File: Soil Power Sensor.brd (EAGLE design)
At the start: 100 x 90 mm, 97 parts, among them IC1 TPD2E2U06DCK, J1 12401832E402A, U1 WIO E5, U10 FSA2466, U12 REF2033, U13 TLV1117LV33, U2 FT234XD, U3 MAX9943ATT+, U4 ESP32-C3-MINI-1-N4, U5 THS4532, U6 LM27761DSG, U7 INA296A5, U8 MAX11201A, X1 SMA-142-0701-801/806

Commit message: Reset board layout
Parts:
- moved C12 216.9 mm to (-105.4, 104.1), turned to 0 degrees
- moved C11 215.2 mm to (-102.9, 116.8), turned to 0 degrees
- moved R27 204.2 mm to (-97.8, 116.8), turned to 0 degrees
- moved R25 203.9 mm to (-87.6, 116.8), turned to 0 degrees
- moved J1 201.6 mm to (-91.4, 7.62), turned to 0 degrees
- moved R15 200.2 mm to (-106.7, 111.8), turned to 0 degrees
- moved R4 199.0 mm to (-101.6, 111.8), turned to 0 degrees
- moved R26 196.2 mm to (-92.7, 116.8), turned to 0 degrees
- moved R24 195.1 mm to (-82.5, 116.8), turned to 0 degrees
- moved TP5 191.9 mm to (-90.2, 120.7)
- moved R23 190.5 mm to (-77.5, 116.8), turned to 0 degrees
- moved C4 186.7 mm to (-91.4, 111.8), turned to 0 degrees
- moved R22 184.0 mm to (-72.4, 116.8), turned to 0 degrees
- moved C7 176.3 mm to (-96.5, 111.8), turned to 0 degrees
- moved JP7 174.4 mm to (-71.1, 86.4), turned to 0 degrees
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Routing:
- net +3V3: track 282.9 -> 0.00 mm, vias 10 -> 0
- net VCC: track 165.2 -> 0.00 mm, vias 4 -> 0
- net N$22: track 95.2 -> 0.00 mm
- net PB3/RTS/JTDO: track 88.2 -> 0.00 mm, vias 2 -> 0
- net PC1: track 79.3 -> 0.00 mm, vias 3 -> 0
- net PC0: track 74.8 -> 0.00 mm, vias 3 -> 0
- net PB4/CTS/JNTRST: track 68.9 -> 0.00 mm, vias 2 -> 0
- net VUSB: track 68.9 -> 0.00 mm, vias 3 -> 0
- net -3V3: track 68.2 -> 0.00 mm, vias 2 -> 0
- net ESP32_TXD0: track 61.6 -> 0.00 mm, vias 2 -> 0
- net ESP32_RXD0: track 60.0 -> 0.00 mm, vias 2 -> 0
- net JTCK: track 47.9 -> 0.00 mm
- net ESP32_NRST: track 45.7 -> 0.00 mm
- net ESP32_EN: track 45.4 -> 0.00 mm, vias 2 -> 0
- net JTMS: track 45.0 -> 0.00 mm
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- removed copper zone on layer 1, net GND
- removed copper zone on layer 15, net GND
- removed copper zone on layer 16, net GND
- removed copper zone on layer 2, net GND
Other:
- board size 100 x 90 mm -> 160 x 100 mm

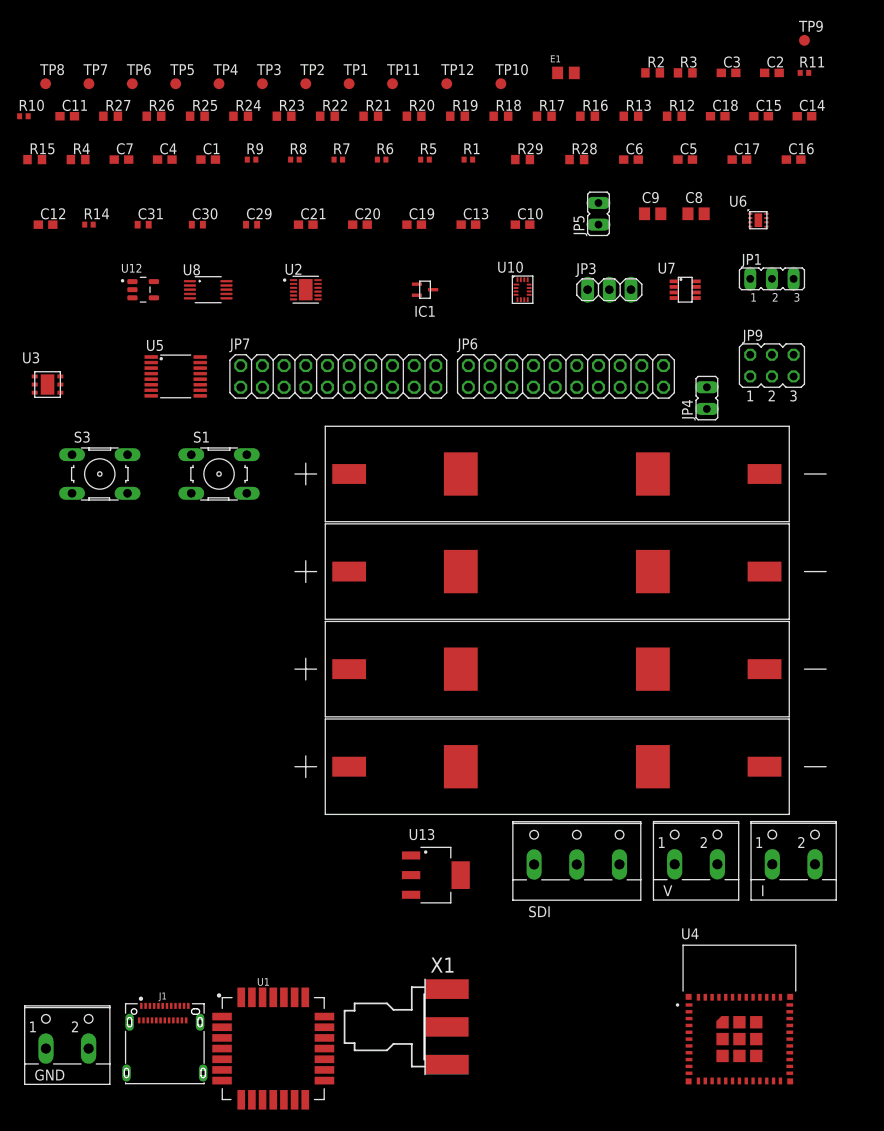
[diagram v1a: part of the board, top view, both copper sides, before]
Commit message: Renumbered all parts
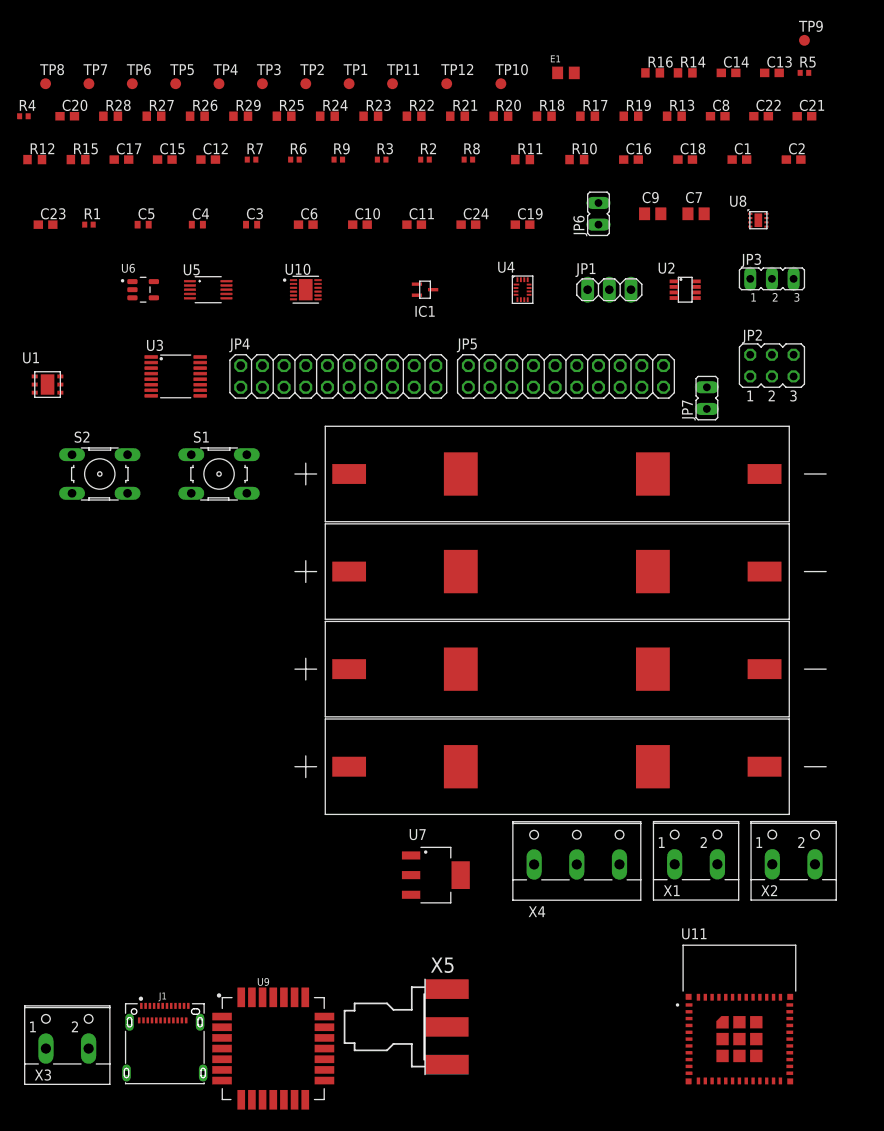
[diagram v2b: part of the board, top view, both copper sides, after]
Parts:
- removed C29, C30, C31: 0.1uF, rcl:C0402
- removed U12: REF2033, Soil Power Sensor:SOT95P280X110-5N
- removed U13: TLV1117LV33, Soil Power Sensor:SOT230P700X180-4N
- removed V: Voltage, con-wago-500:W237-102
- added C22: NC, rcl:C0603
- added C23: 10uF, rcl:C0603
- added C24: 0.1uF, rcl:C0603
- added U11: ESP32-C3-MINI-1-N4, Soil Power Sensor:XCVR_ESP32-C3-MINI-1-N4
- added U9: WIO E5, Soil Power Sensor:MODULE28P-1.25-12X12X2.5MM
- added X5: SMA-142-0701-801/806, con-coax:J502-ND-142-0701-801/806
- C1: value 4.7u -> 16uF
- C10: value 0.1uF -> 4.7uF
- C11: value 1uF -> 2.2uF
- C12: value 10uF -> 4.7u
- C13: value 0.1uF -> NC
- C15: value NC -> 0.1u
- C16: value 20uF -> 100n
- C17: value 16uF -> 4.7u
- C18: value 1uF -> 100n
- C19: value 2.2uF -> 0.1uF
- C2: value NC -> 20uF
- C20: value 4.7uF -> 1uF
- C21: value 4.7uF -> NC
- C3: value NC -> 0.1uF; device rcl:C0603 -> rcl:C0402
- C4: value 0.1u -> 0.1uF; device rcl:C0603 -> rcl:C0402
- C5: value 100n -> 0.1uF; device rcl:C0603 -> rcl:C0402
- C6: value 100n -> 4.7uF
- C7: value 4.7u -> 1uF; device rcl:C0603 -> rcl:C0805
- C8: device rcl:C0805 -> rcl:C0603
- JP1: value Power Mode -> Rsense; device jumper:JP2 -> pinhead:1X03
- JP3: value Rsense -> Power Mode; device pinhead:1X03 -> jumper:JP2
- JP4: value Boot Option -> STM32 JTAG; device jumper:JP1 -> pinhead:2X10
- JP5: value USB -> ESP32 JTAG; device jumper:JP1 -> pinhead:2X10
- JP6: value ESP32 JTAG -> USB; device pinhead:2X10 -> jumper:JP1
- JP7: value STM32 JTAG -> Boot Option; device pinhead:2X10 -> jumper:JP1
- R1: value 100k -> 330m
- R10: value 10k -> 169k; device rcl:R0402 -> rcl:R0603
- R11: value 10k -> 100k; device rcl:R0402 -> rcl:R0603
- R12: value 1M -> 5.1k
- R13: value 0 -> 1M
- R14: value 330m -> 1M; device rcl:R0402 -> rcl:R0603
- R2: value 0 -> 100k; device rcl:R0603 -> rcl:R0402
- R23, R24: value 10k -> 0
- R26: value 0 -> 10k
- R28: value 169k -> 0
- R29, R5: value 100k -> 10k
- R3: value 1M -> 100k; device rcl:R0603 -> rcl:R0402
- R4: value 5.1k -> 10k; device rcl:R0603 -> rcl:R0402
- R6, R7: value 100k -> 250k
- R8, R9: value 250k -> 100k
- U1: value WIO E5 -> MAX9943ATT+; device Soil Power Sensor:MODULE28P-1.25-12X12X2.5MM -> Soil Power Sensor:TDFN300X300X75-6N
- U10: value FSA2466 -> FT234XD; device Soil Power Sensor:UQFN40P180X260X50-16N -> Soil Power Sensor:SON45P300X300X80-13N
- U2: value FT234XD -> INA296A5; device Soil Power Sensor:SON45P300X300X80-13N -> Soil Power Sensor:SOT65P280X110-8N
- U3: value MAX9943ATT+ -> THS4532; device Soil Power Sensor:TDFN300X300X75-6N -> Soil Power Sensor:SOP65P640X120-16N
- U4: value ESP32-C3-MINI-1-N4 -> FSA2466; device Soil Power Sensor:XCVR_ESP32-C3-MINI-1-N4 -> Soil Power Sensor:UQFN40P180X260X50-16N
- U5: value THS4532 -> MAX11201A; device Soil Power Sensor:SOP65P640X120-16N -> Soil Power Sensor:SOP50P490X110-10N
- U6: value LM27761DSG -> REF2033; device Soil Power Sensor:SON50P200X200X80-9TPN -> Soil Power Sensor:SOT95P280X110-5N
- U7: value INA296A5 -> TLV1117LV33; device Soil Power Sensor:SOT65P280X110-8N -> Soil Power Sensor:SOT230P700X180-4N
- U8: value MAX11201A -> LM27761DSG; device Soil Power Sensor:SOP50P490X110-10N -> Soil Power Sensor:SON50P200X200X80-9TPN
- X1: value SMA-142-0701-801/806 -> Voltage; device con-coax:J502-ND-142-0701-801/806 -> con-wago-500:W237-102
- moved U4 88.8 mm to (-49.5, 96.5)
- moved U1 83.6 mm to (-106.7, 86.4)
- moved R12 75.1 mm to (-106.7, 111.8)
- moved U7 74.5 mm to (-59.7, 27.9)
- moved C17 72.4 mm to (-96.5, 111.8)
- moved R14 72.1 mm to (-30.5, 121.9)
- moved U6 71.7 mm to (-94.0, 96.5)
- moved C15 70.0 mm to (-91.4, 111.8)
- moved C7 67.6 mm to (-29.2, 105.4)
- moved R10 65.0 mm to (-43.2, 111.8)
- moved U8 64.1 mm to (-22.9, 105.4)
- moved C5 64.0 mm to (-94.0, 104.1)
- moved C1 62.2 mm to (-24.1, 111.8)
- moved C21 59.8 mm to (-16.5, 116.8)
- moved C3 58.6 mm to (-81.3, 104.1)
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- renumbered GND to X3, I to X2, JP9 to JP2, S3 to S2, SDI to X4
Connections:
- net +3V3: now also C23.1, C24.1, JP4.1, JP4.2, JP5.1, JP5.2, R26.2, R29.2, U1.6, U11.3, U2.6, U3.13, U3.9, U4.14, U5.6, U5.7, U7.2, U7.4, U9.1; no longer C1.1, C13.1, JP6.1, JP6.2, JP7.1, JP7.2, R24.2, R25.2, U1.1, U10.14, U13.2, U13.4, U3.6, U4.3, U5.13, U5.9, U7.6, U8.6, U8.7
- net -3V3: now also C11.1, R10.2, U1.2, U8.4; no longer C19.1, R28.2, U3.2, U6.4
- net CURRENT_N: now also C1.1, R6.2, U3.11, U4.15; no longer C17.1, R8.2, U10.15, U5.11
- net CURRENT_P: now also C1.2, R7.2, U3.10, U4.3; no longer C17.2, R9.2, U10.3, U5.10
- net D_N: now also R27.1, U11.26; no longer R26.1, U4.26
- net D_P: now also R28.1, U11.27; no longer R27.1, U4.27
- net ESP32_EN: now also R25.2, U9.21; no longer R23.2, U1.21
- net ESP32_NRST: now also C19.1, JP5.15, R24.1; no longer C10.1, JP6.15, R22.1
- net ESP32_RXD0: now also U11.30, U9.18; no longer U1.18, U4.30
- net ESP32_TXD0: now also U11.31, U9.19; no longer U1.19, U4.31
- net GND: now also C16.2, C17.2, C18.2, C22.2, C23.2, C24.2, C3.1, C7.1, G1.N1, G1.N2, JP4.10, JP4.12, JP4.14, JP4.16, JP4.18, JP4.20, JP4.4, JP4.6, JP4.8, JP5.10, JP5.12, JP5.14, JP5.16, JP5.18, JP5.20, JP5.4, JP5.6, JP5.8, JP7.2, R11.1, R12.1, R14.1, R15.2, U10.13, U10.5, U11.1, U11.11, U11.14, U11.2, U11.36, U11.37, U11.38, U11.39, U11.40, U11.41, U11.42, U11.43, U11.44, U11.45, U11.46, U11.47, U11.48, U11.49_1, U11.49_2, U11.49_3, U11.49_4, U11.49_5, U11.49_6, U11.49_7, U11.49_8, U11.49_9, U11.50, U11.51, U11.52, U11.53, U2.2, U3.12, U3.16, U4.6, U5.1, U5.3, U7.1, U8.2, U8.9, U9.14, U9.16, U9.2, U9.22, X5.G@1, X5.G@2, X5.G@3, X5.G@4; no longer C1.2, C2.2, C29.1, C3.2, C30.2, C31.2, C7.2, C8.1, G4.N1, G4.N2, JP4.2, JP6.10, JP6.12, JP6.14, JP6.16, JP6.18, JP6.20, JP6.4, JP6.6, JP6.8, JP7.10, JP7.12, JP7.14, JP7.16, JP7.18, JP7.20, JP7.4, JP7.6, JP7.8, R15.1, R29.1, R3.1, R4.2, U1.14, U1.16, U1.2, U1.22, U10.6, U12.2, U13.1, U2.13, U2.5, U4.1, U4.11, U4.14, U4.2, U4.36, U4.37, U4.38, U4.39, U4.40, U4.41, U4.42, U4.43, U4.44, U4.45, U4.46, U4.47, U4.48, U4.49_1, U4.49_2, U4.49_3, U4.49_4, U4.49_5, U4.49_6, U4.49_7, U4.49_8, U4.49_9, U4.50, U4.51, U4.52, U4.53, U5.12, U5.16, U6.9, U7.2, U8.1, U8.3, X1.G@1, X1.G@2, X1.G@3, X1.G@4
- net IO4/TMS: now also JP5.7, U11.18; no longer JP6.7, U4.18
- net IO5/TDI: now also JP5.5, U11.19; no longer JP6.5, U4.19
- net IO6/TCK: now also JP5.9, U11.20; no longer JP6.9, U4.20
- net IO7/TDO: now also JP5.13, U11.21; no longer JP6.13, U4.21
- net IO9/BOOT: now also JP7.1, U11.23; no longer JP4.1, U4.23
- net JTCK: now also JP4.9, U9.4; no longer JP7.9, U1.4
- net JTDI: now also JP4.5, U9.6; no longer JP7.5, U1.6
- net JTMS: now also JP4.7, U9.3; no longer JP7.7, U1.3
- net N$1: now also U1.3, X1.1; no longer U3.3, V.1
- net N$10: now also R20.1, U10.8; no longer R18.1, U2.8
- net N$11: now also R21.1, U10.11; no longer R19.1, U2.11
- net N$12: now also R22.1, U10.10; no longer R20.1, U2.10
- net N$13: now also R23.1, U10.7; no longer R21.1, U2.7
- net N$14: now also C18.1, U10.2, U10.3, U10.9; no longer C5.1, U2.2, U2.3, U2.9
- net N$15: now also C16.1, C17.1, U10.4; no longer C6.1, C7.1, U2.4
- net N$16: now also G3.P1, G3.P2, G4.N1, G4.N2; no longer G1.N1, G1.N2, G2.P1, G2.P2
- net N$17: now also G2.P1, G2.P2, G3.N1, G3.N2; no longer G2.N1, G2.N2, G3.P1, G3.P2
- net N$18: now also G1.P1, G1.P2, G2.N1, G2.N2; no longer G3.N1, G3.N2, G4.P1, G4.P2
- net N$19: now also G4.P1, G4.P2, JP3.3; no longer G1.P1, G1.P2, JP1.3
- net N$2: now also C14.1, R16.2, X5.1; no longer C3.1, R2.2, X1.1
- net N$21: now also R29.1, U11.22; no longer R24.1, U4.22
- net N$22: now also U9.23; no longer U1.23
- net N$24: now also C20.1, R24.2, R25.1, U11.8; no longer C11.1, R22.2, R23.1, U4.8
- net N$25: now also R26.1, U11.5; no longer R25.1, U4.5
- net N$29: now also R2.2, R8.1, U3.2; no longer R1.1, R5.2, U5.2
- net N$3: now also C13.1, R16.1, U9.15; no longer C2.1, R2.1, U1.15
- net N$30: now also R3.2, R9.1, U3.3; no longer R6.2, R7.1, U5.3
- net N$32: now also C8.1, U8.7; no longer C18.1, U6.7
- net N$33: now also R4.2, R6.1, U3.6; no longer R10.2, R8.1, U5.6
- net N$34: now also R13.1, R14.2, U9.27; no longer R12.1, R3.2, U1.27
- net N$36: now also R5.2, R7.1, U3.7; no longer R11.2, R9.1, U5.7
- net N$37: now also R4.1, U2.5; no longer R10.1, U7.5
- net N$38: now also JP1.3, R1.1, U2.1; no longer JP3.3, R14.1, U7.1
- net N$39: now also C21.1, JP6.1, R27.2; no longer C14.1, JP5.1, R26.2
- net N$40: now also C22.1, JP6.2, R28.2; no longer C15.1, JP5.2, R27.2
- net N$41: now also U4.16, U5.4; no longer U10.16, U8.4
- net N$42: now also U4.4, U5.5; no longer U10.4, U8.5
- net N$44: now also R10.1, R11.2, U8.5; no longer R28.1, R29.2, U6.5
- net N$45: now also R1.2, U2.8; no longer R14.2, U7.8
- net N$46: now also R3.1, X1.2; no longer R6.1, V.2
- net N$48: now also JP1.1; no longer JP3.1
- net N$5: now also C8.2, U8.8; no longer C18.2, U6.8
- net N$53: now also C10.1, U8.3; no longer C20.1, U6.3
- net N$6: now also R12.2; no longer R15.2
- net N$7: now also R15.1; no longer R4.1
- net N$8: now also R2.1, U1.1, U1.4; no longer R5.1, U3.1, U3.4
- net NRST: now also JP4.15, R19.2; no longer JP7.15, R13.2
- net PB13/SPI2_SCK: now also U5.9, U9.24; no longer U1.24, U8.9
- net PB14/SPI2_MISO: now also U5.8, U9.26; no longer U1.26, U8.8
- net PB3/RTS/JTDO: now also JP4.13, R20.2, U9.8; no longer JP7.13, R18.2, U1.8
- net PB4/CTS/JNTRST: now also JP4.3, R21.2, U9.7; no longer JP7.3, R19.2, U1.7
- net PB6/TX: now also R23.2, U9.10; no longer R21.2, U1.10
- net PB7/RX: now also R22.2, U9.9; no longer R20.2, U1.9
- net PB9/SPI2_NSS: now also U4.2, U9.25; no longer U1.25, U10.2
- net PC0: now also U3.1, U3.5, U9.13; no longer U1.13, U5.1, U5.5
- net PC1: now also U6.3, U8.6, U9.12; no longer U1.12, U12.3, U6.6
- net REF+1V65: now also C4.1, R5.1, U2.3, U2.7, U3.4, U3.8, U6.1; no longer C30.1, R11.1, U12.1, U5.4, U5.8, U7.3, U7.7
- net REF+3V3: now also C5.1, U5.2, U6.5; no longer C31.1, U12.5, U8.2
- net RST: now also C15.1, R19.1, U9.17; no longer C4.1, R13.1, U1.17
- net STMR_D_N: now also R18.2, U10.1; no longer R17.2, U2.1
- net STMR_D_P: now also R17.2, U10.12; no longer R16.2, U2.12
- net STM_D_N: now also R18.1; no longer R17.1
- net STM_D_P: now also R17.1; no longer R16.1
- net VCC: now also C3.2, C6.1, C7.2, JP3.2, R13.2, U6.4, U7.3, U8.1; no longer C21.1, C29.2, C8.2, JP1.2, R12.2, U12.4, U13.3, U6.1
- net VOLTAGE_N: now also C2.2, R8.2, U3.15, U4.1; no longer C16.2, R1.2, U10.1, U5.15
- net VOLTAGE_P: now also C2.1, R9.2, U3.14, U4.5; no longer C16.1, R7.2, U10.5, U5.14
- net VUSB: now also JP3.1; no longer JP1.1

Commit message: Redesigned board
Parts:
- removed TP1, TP10, TP11, TP12, TP2, TP3, TP4, TP5, TP6, TP7, TP8, TP9: TPB1,27, testpad:B1,27
- added I, IN, IP, VBUF, VCM, VN, VP: TPB1,27, testpad:B1,27
- moved C23 215.0 mm to (91.4, 17.8)
- moved R28 208.2 mm to (76.2, 2.54), turned to 180 degrees
- moved R27 202.5 mm to (76.2, 5.08), turned to 180 degrees
- moved C20 201.6 mm to (78.7, 29.2), turned to 180 degrees
- moved R26 195.8 mm to (81.3, 17.8), turned to 180 degrees
- moved S2 192.3 mm to (86.4, 24.1)
- moved R12 191.6 mm to (78.7, 63.5)
- moved R29 191.3 mm to (76.2, 10.2), turned to 90 degrees
- moved J1 188.1 mm to (88.9, 61.0), turned to 90 degrees
- moved R15 187.4 mm to (78.7, 61.0), turned to 180 degrees
- moved C15 186.9 mm to (73.7, 24.1), turned to 270 degrees
- moved R25 181.0 mm to (78.7, 25.4), turned to 180 degrees
- moved R24 179.1 mm to (83.8, 29.2), turned to 180 degrees
- moved C17 175.9 mm to (71.1, 58.4)
- moved S1 173.1 mm to (86.4, 50.8), turned to 180 degrees
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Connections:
- net +3V3: no longer TP2.TP
- net -3V3: no longer TP1.TP
- net CURRENT_N: now also IN.TP; no longer TP10.TP
- net CURRENT_P: now also IP.TP; no longer TP11.TP
- net N$37: now also I.TP; no longer TP12.TP
- net N$46: now also VCM.TP; no longer TP6.TP
- net N$8: now also VBUF.TP; no longer TP7.TP
- net REF+1V65: no longer TP4.TP
- net REF+3V3: no longer TP3.TP
- net VCC: no longer TP5.TP
- net VOLTAGE_N: now also VN.TP; no longer TP8.TP
- net VOLTAGE_P: now also VP.TP; no longer TP9.TP
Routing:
- net +3V3: track 0.00 -> 230.8 mm, vias 0 -> 11
- net VCC: track 0.00 -> 167.8 mm, vias 0 -> 3
- net VUSB: track 0.00 -> 119.2 mm, vias 0 -> 1
- net ESP32_NRST: track 0.00 -> 92.6 mm
- net N$22: track 0.00 -> 86.7 mm, vias 0 -> 2
- net PB3/RTS/JTDO: track 0.00 -> 79.8 mm, vias 0 -> 3
- net N$46: track 0.00 -> 73.5 mm, vias 0 -> 2
- net PC1: track 0.00 -> 70.4 mm, vias 0 -> 2
- net PC0: track 0.00 -> 62.1 mm, vias 0 -> 4
- net N$38: track 0.00 -> 58.9 mm, vias 0 -> 1
- net IO7/TDO: track 0.00 -> 57.7 mm, vias 0 -> 1
- net PB9/SPI2_NSS: track 0.00 -> 53.4 mm, vias 0 -> 2
- net IO6/TCK: track 0.00 -> 52.3 mm, vias 0 -> 1
- net N$1: track 0.00 -> 50.2 mm
- net PB4/CTS/JNTRST: track 0.00 -> 50.0 mm, vias 0 -> 2
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- added copper zone on layer 1, net GND
- added copper zone on layer 15, net GND
- added copper zone on layer 16, net GND
- added copper zone on layer 2, net GND
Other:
- board size 160 x 100 mm -> 94 x 67 mm
- board text added: "Name"
- board text added: "Soil Power Sensor >REVISION John Madden UC Santa Cruz >DATE"
